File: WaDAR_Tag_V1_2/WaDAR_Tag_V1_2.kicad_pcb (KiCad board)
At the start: 2 copper layers, 34.6 x 30.7 mm, 11 parts, among them J1 SMA-J-P-H-RA-TH1, U1 SiT1569

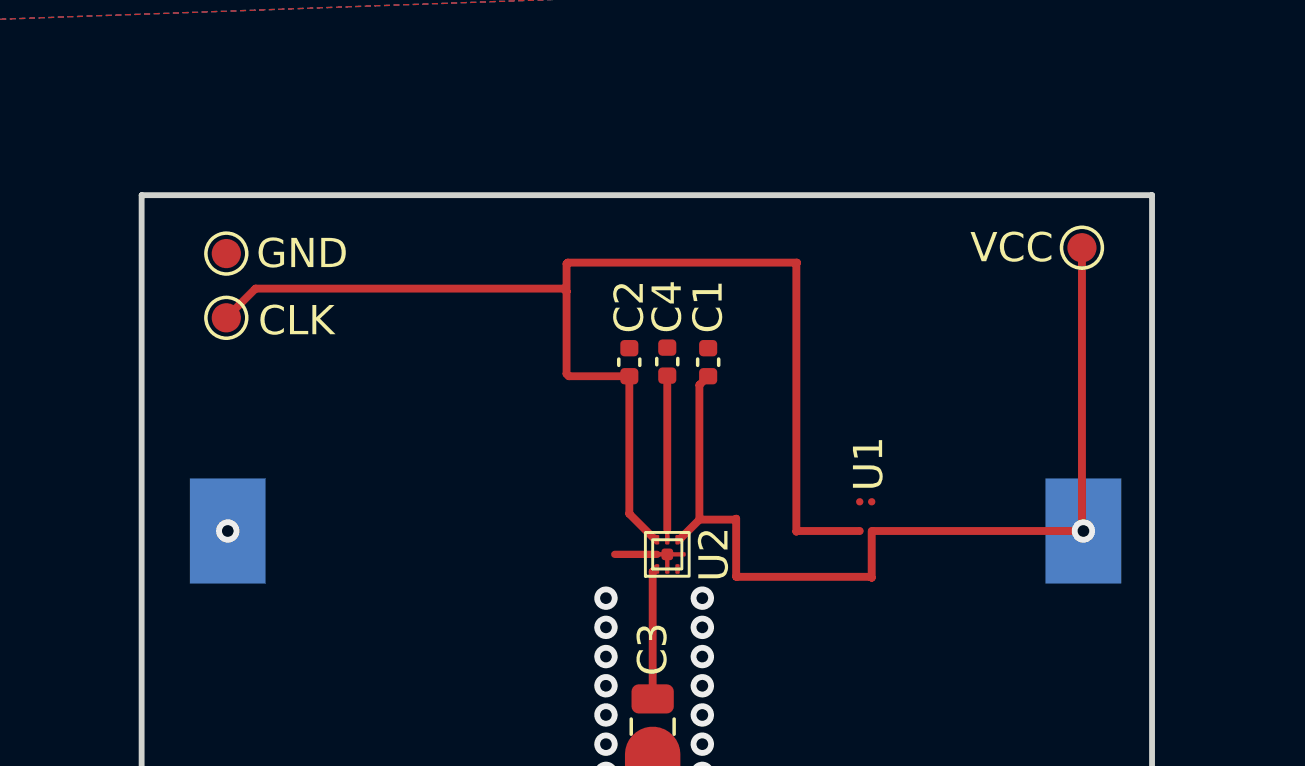
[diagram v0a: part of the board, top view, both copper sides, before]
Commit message: updated datasheets
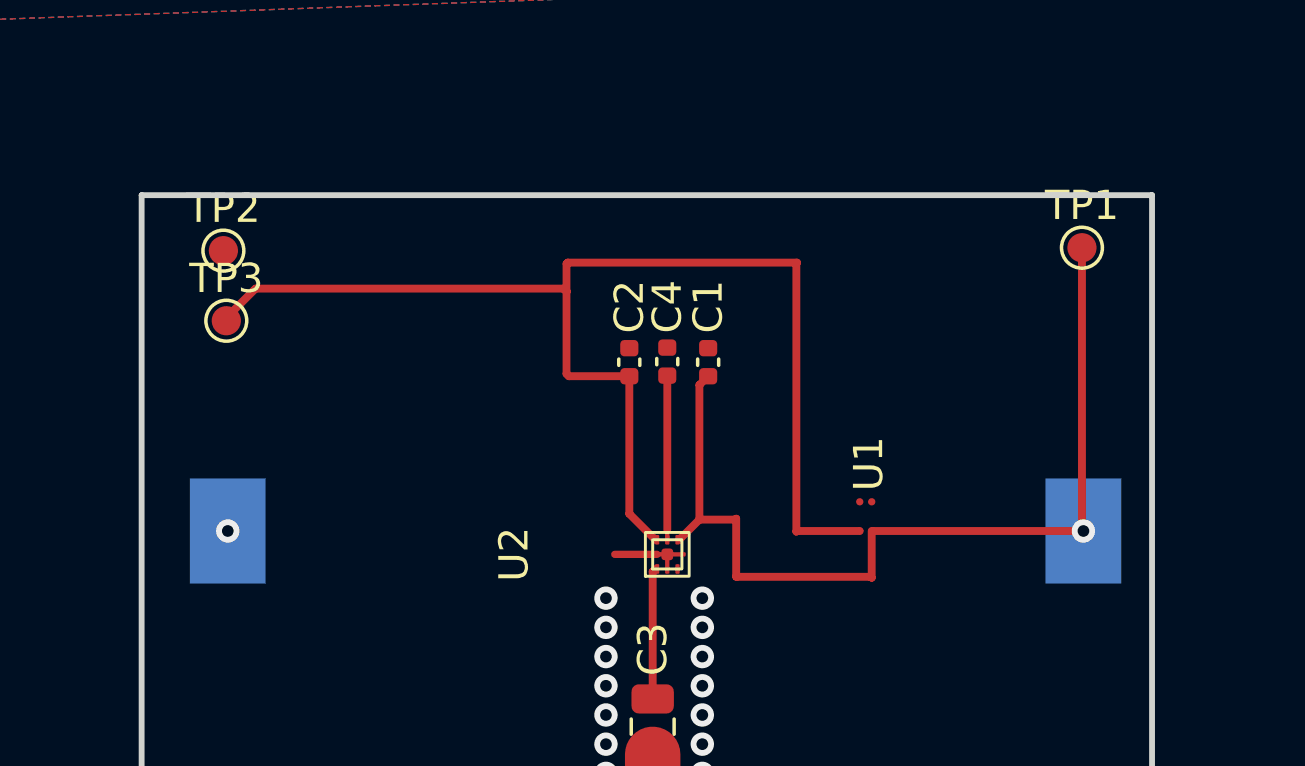
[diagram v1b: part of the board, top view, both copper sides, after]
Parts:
- removed CLK: CLK, TestPoint:TestPoint_Pad_D1.0mm
- removed GND: GND, TestPoint:TestPoint_Pad_D1.0mm
- removed VCC: VCC, TestPoint:TestPoint_Pad_D1.0mm
- added TP1: VCC, TestPoint:TestPoint_Pad_D1.0mm, F.Cu at (178.2, 47.3)
- added TP2: GND, TestPoint:TestPoint_Pad_D1.0mm, F.Cu at (148.8, 47.4)
- added TP3: CLK, TestPoint:TestPoint_Pad_D1.0mm, F.Cu at (148.9, 49.8)
- U2: footprint JLab_FP:SKY13351_FP -> Library:SKY13351_FP
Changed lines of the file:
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@@
 	(footprint "TestPoint:TestPoint_Pad_D1.0mm"
 		(layer "F.Cu")
-		(at 148.9 47.5)
+		(at 148.8 47.4)
 		(descr "SMD pad as test Point, diameter 1.0mm")
 		(tags "test point SMD pad")
-		(property "Reference" "GND"
-			(at 2.6 0 0)
+		(property "Reference" "TP2"
+			(at 0 -1.448 0)
 			(layer "F.SilkS")
 			(effects
@@
 			(layers "F.Cu" "F.Mask")
 			(net 1 "GND")
-			(pinfunction "1")
-			(pintype "passive")
-		)
-	)
-	(footprint "TestPoint:TestPoint_Pad_D1.0mm"
-		(layer "F.Cu")
-		(at 148.9 49.7)
-		(descr "SMD pad as test Point, diameter 1.0mm")
-		(tags "test point SMD pad")
-		(property "Reference" "CLK"
-			(at 2.4 0.1 0)
-			(layer "F.SilkS")
-			(effects
-				(font
-					(size 1 1)
-					(thickness 0.15)
-				)
-			)
-		)
-		(property "Value" "CLK"
-			(at 0 1.55 0)
-			(layer "F.Fab")
-			(effects
-				(font
-					(size 1 1)
-					(thickness 0.15)
-				)
-			)
-		)
-		(property "Footprint" "TestPoint:TestPoint_Pad_D1.0mm"
-			(at 0 0 0)
-			(layer "F.Fab")
-			(hide yes)
-			(effects
-				(font
-					(size 1.27 1.27)
-					(thickness 0.15)
-				)
-			)
-		)
-		(property "Datasheet" ""
-			(at 0 0 0)
-			(layer "F.Fab")
-			(hide yes)
-			(effects
-				(font
-					(size 1.27 1.27)
-					(thickness 0.15)
-				)
-			)
-		)
-		(property "Description" "test point"
-			(at 0 0 0)
-			(layer "F.Fab")
-			(hide yes)
-			(effects
-				(font
-					(size 1.27 1.27)
-					(thickness 0.15)
-				)
-			)
-		)
-		(property ki_fp_filters "Pin* Test*")
-		(sheetname "Root")
-		(sheetfile "WaDAR_Tag_V1_2.kicad_sch")
-		(attr exclude_from_pos_files)
-		(fp_circle
-			(center 0 0)
-			(end 0 0.7)
-			(stroke
-				(width 0.12)
-				(type solid)
-			)
-			(fill none)
-			(layer "F.SilkS")
-		)
-		(fp_circle
-			(center 0 0)
-			(end 1 0)
-			(stroke
-				(width 0.05)
-				(type solid)
-			)
-			(fill none)
-			(layer "F.CrtYd")
-		)
-		(fp_text user "${REFERENCE}"
-			(at 0 -1.45 0)
-			(layer "F.Fab")
-			(effects
-				(font
-					(size 1 1)
-					(thickness 0.15)
-				)
-			)
-		)
-		(pad "1" smd circle
-			(at 0 0)
-			(size 1 1)
-			(layers "F.Cu" "F.Mask")
-			(net 3 "Net-(U1-CLK_Out)")
 			(pinfunction "1")
 			(pintype "passive")
@@
 		(descr "SMD pad as test Point, diameter 1.0mm")
 		(tags "test point SMD pad")
-		(property "Reference" "VCC"
-			(at -2.4 0 0)
+		(property "Reference" "TP1"
+			(at 0 -1.448 0)
 			(layer "F.SilkS")
 			(effects
@@
 		)
 	)
-	(footprint "JLab_FP:SKY13351_FP"
+	(footprint "TestPoint:TestPoint_Pad_D1.0mm"
+		(layer "F.Cu")
+		(at 148.9 49.8)
+		(descr "SMD pad as test Point, diameter 1.0mm")
+		(tags "test point SMD pad")
+		(property "Reference" "TP3"
+			(at 0 -1.448 0)
+			(layer "F.SilkS")
+			(effects
+				(font
+					(size 1 1)
+					(thickness 0.15)
+				)
+			)
+		)
+		(property "Value" "CLK"
+			(at 0 1.55 0)
+			(layer "F.Fab")
+			(effects
+				(font
+					(size 1 1)
+					(thickness 0.15)
+				)
+			)
+		)
+		(property "Footprint" "TestPoint:TestPoint_Pad_D1.0mm"
+			(at 0 0 0)
+			(layer "F.Fab")
+			(hide yes)
+			(effects
+				(font
+					(size 1.27 1.27)
+					(thickness 0.15)
+				)
+			)
+		)
+		(property "Datasheet" ""
+			(at 0 0 0)
+			(layer "F.Fab")
+			(hide yes)
+			(effects
+				(font
+					(size 1.27 1.27)
+					(thickness 0.15)
+				)
+			)
+		)
+		(property "Description" "test point"
+			(at 0 0 0)
+			(layer "F.Fab")
+			(hide yes)
+			(effects
+				(font
+					(size 1.27 1.27)
+					(thickness 0.15)
+				)
+			)
+		)
+		(property ki_fp_filters "Pin* Test*")
+		(sheetname "Root")
+		(sheetfile "WaDAR_Tag_V1_2.kicad_sch")
+		(attr exclude_from_pos_files)
+		(fp_circle
+			(center 0 0)
+			(end 0 0.7)
+			(stroke
+				(width 0.12)
+				(type solid)
+			)
+			(fill none)
+			(layer "F.SilkS")
+		)
+		(fp_circle
+			(center 0 0)
+			(end 1 0)
+			(stroke
+				(width 0.05)
+				(type solid)
+			)
+			(fill none)
+			(layer "F.CrtYd")
+		)
+		(fp_text user "${REFERENCE}"
+			(at 0 -1.45 0)
+			(layer "F.Fab")
+			(effects
+				(font
+					(size 1 1)
+					(thickness 0.15)
+				)
+			)
+		)
+		(pad "1" smd circle
+			(at 0 0)
+			(size 1 1)
+			(layers "F.Cu" "F.Mask")
+			(net 3 "Net-(U1-CLK_Out)")
+			(pinfunction "1")
+			(pintype "passive")
+		)
+	)
+	(footprint "Library:SKY13351_FP"
 		(layer "F.Cu")
 		(at 159.25 57.8 90)
 		(property "Reference" "U2"
-			(at 0 6.35 90)
+			(at 0 -0.5 90)
 			(unlocked yes)
 			(layer "F.SilkS")
@@
 				(font
 					(size 1 1)
-					(thickness 0.15)
+					(thickness 0.1)
 				)
 			)
@@
 			(unlocked yes)
 			(layer "F.Fab")
-			(hide yes)
-			(effects
-				(font
-					(size 1 1)
-					(thickness 0.15)
-				)
-			)
-		)
-		(property "Footprint" "JLab_FP:SKY13351_FP"
+			(effects
+				(font
+					(size 1 1)
+					(thickness 0.15)
+				)
+			)
+		)
+		(property "Footprint" "Library:SKY13351_FP"
 			(at 0 0 90)
 			(layer "F.Fab")
